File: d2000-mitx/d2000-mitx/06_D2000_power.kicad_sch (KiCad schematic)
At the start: 2 parts

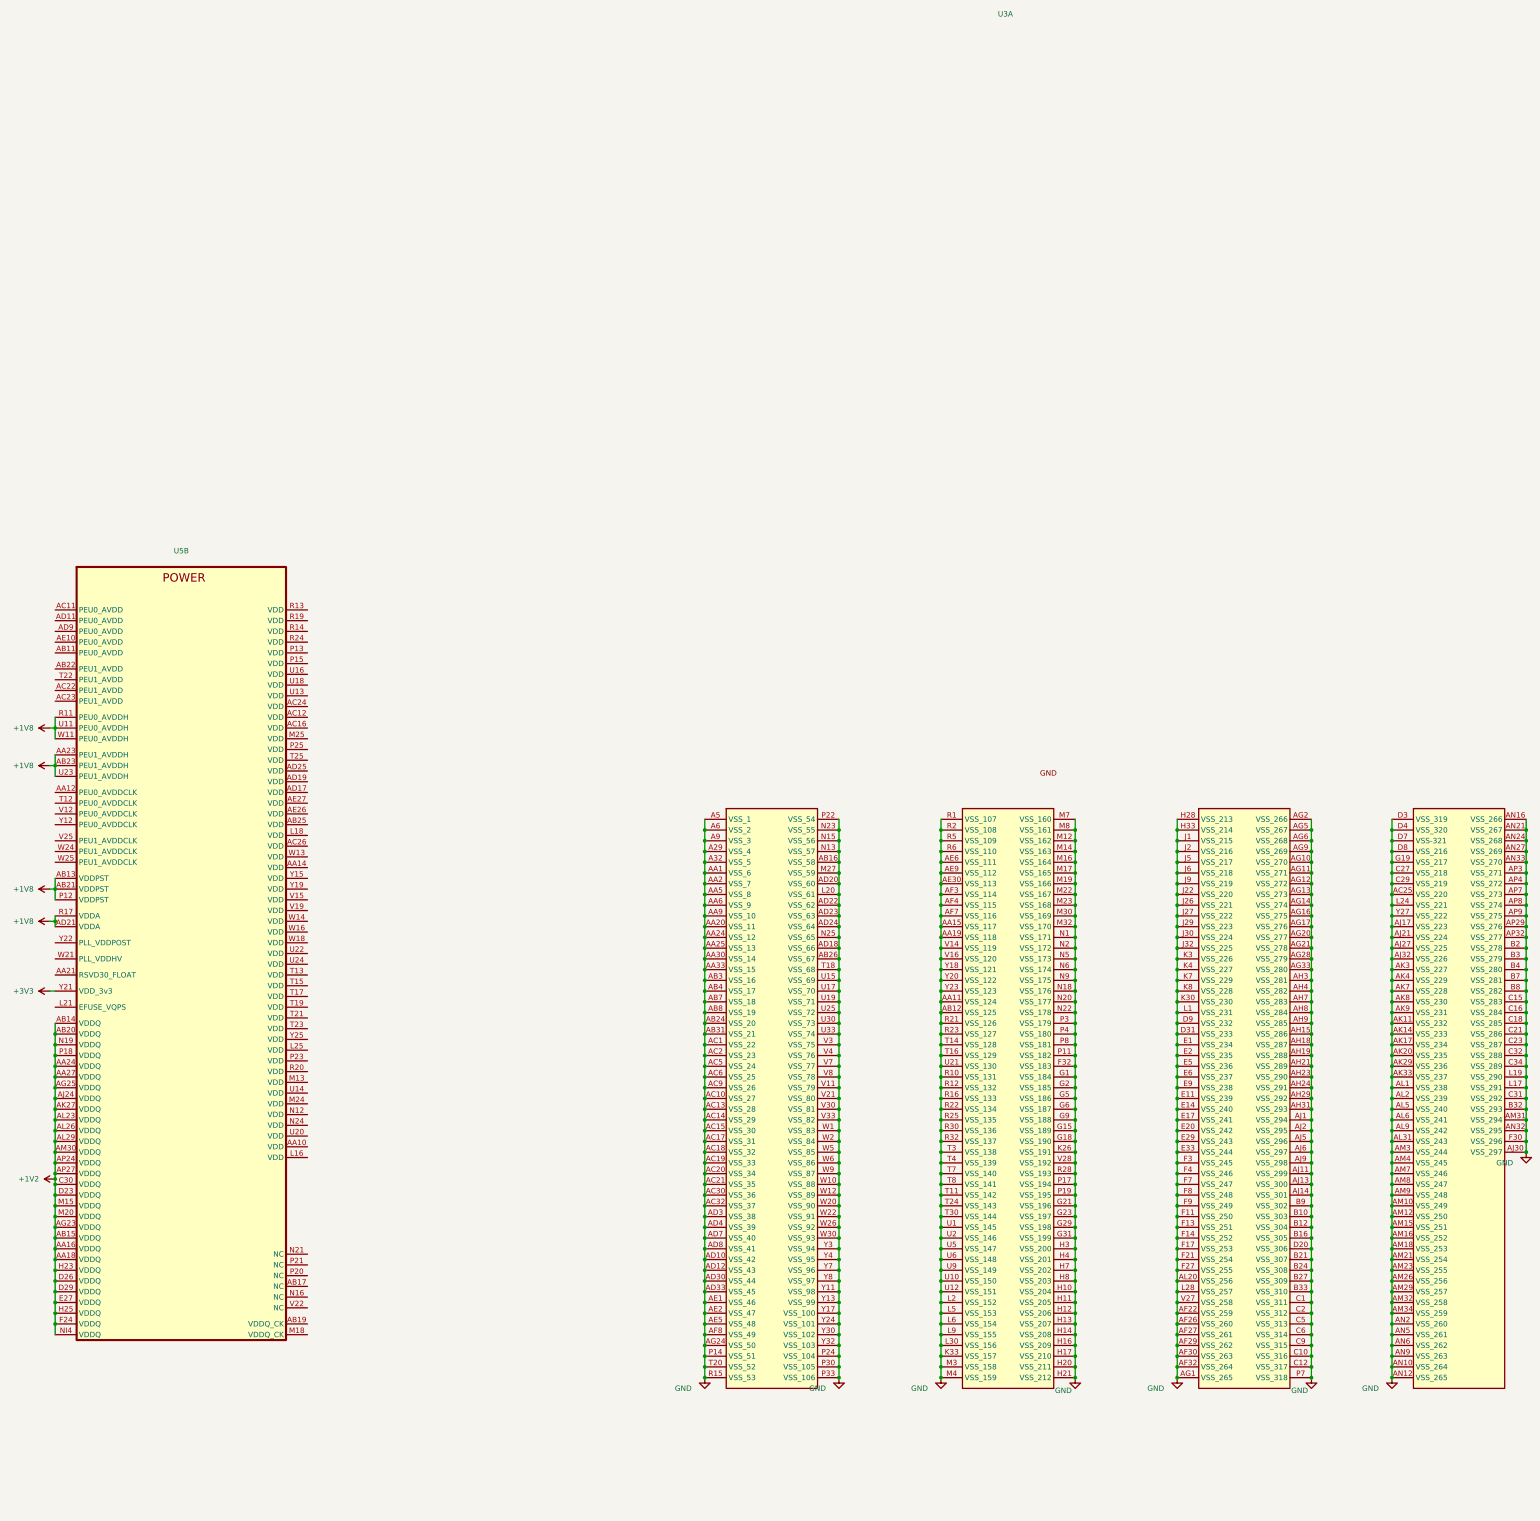
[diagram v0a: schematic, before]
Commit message: update schem + pcb layout
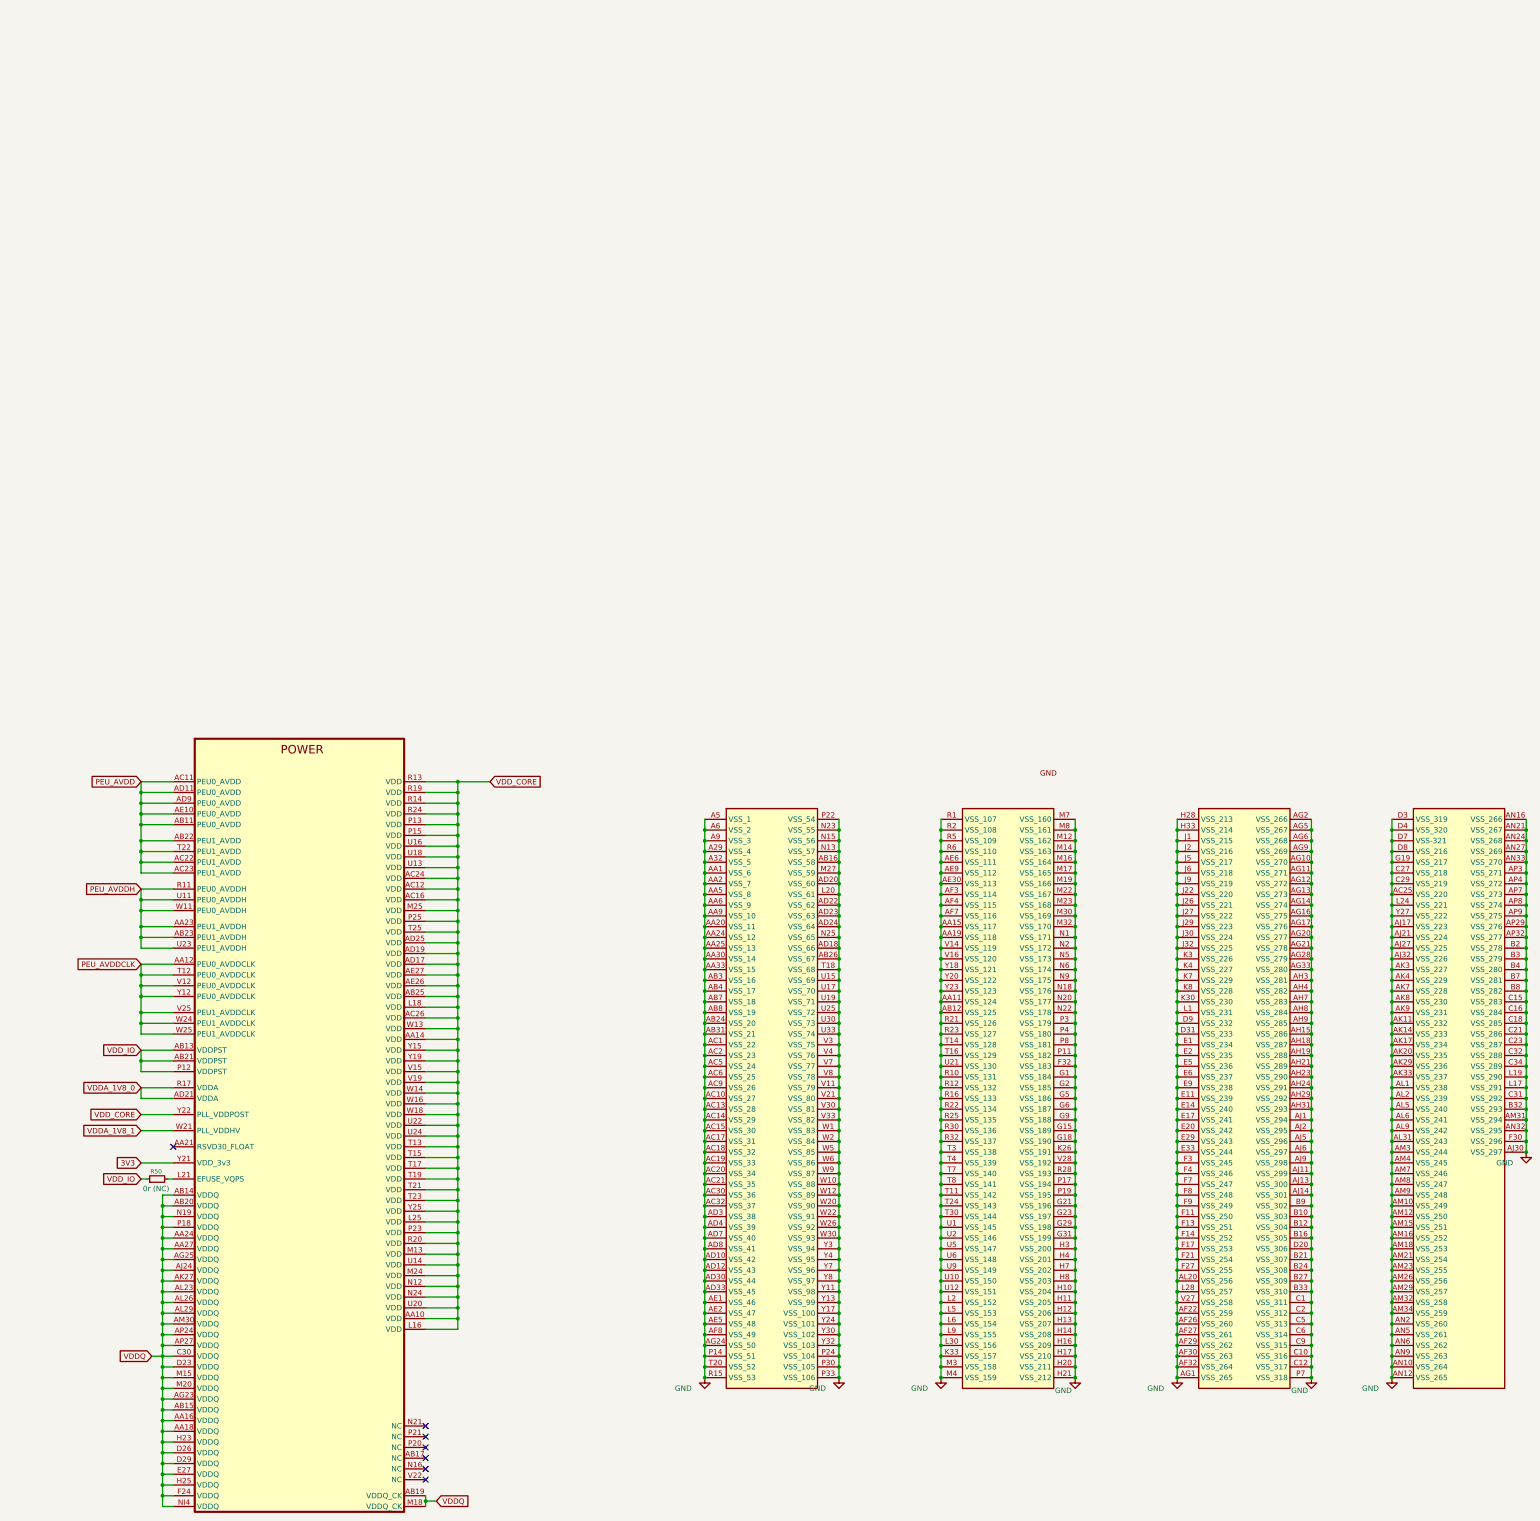
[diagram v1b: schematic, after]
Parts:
- removed U3, U5: ~, symbol D2000:D2000-E8
- added R50: 0r (NC), Resistor_SMD:R_0402_1005Metric, symbol Device:R_Small
- added U5: ~, D2000:D2000_DDR4_BGA1144P100_3500X350, symbol D2000-FT20004:D2000-E8
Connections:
- net GND: now also U5.A29 (VSS_4), U5.A32 (VSS_5), U5.A5 (VSS_1), U5.A6 (VSS_2), U5.A9 (VSS_3), U5.AA1 (VSS_6), U5.AA11 (VSS_124), U5.AA15 (VSS_117), U5.AA19 (VSS_118), U5.AA2 (VSS_7), U5.AA20 (VSS_11), U5.AA24 (VSS_12), U5.AA25 (VSS_13), U5.AA30 (VSS_14), U5.AA33 (VSS_15), U5.AA5 (VSS_8), U5.AA6 (VSS_9), U5.AA9 (VSS_10), U5.AB12 (VSS_125), U5.AB16 (VSS_58), U5.AB24 (VSS_20), U5.AB26 (VSS_67), U5.AB3 (VSS_16), U5.AB31 (VSS_21), U5.AB4 (VSS_17), U5.AB7 (VSS_18), U5.AB8 (VSS_19), U5.AC1 (VSS_22), U5.AC10 (VSS_27), U5.AC13 (VSS_28), U5.AC14 (VSS_29), U5.AC15 (VSS_30), U5.AC17 (VSS_31), U5.AC18 (VSS_32), U5.AC19 (VSS_33), U5.AC2 (VSS_23), U5.AC20 (VSS_34), U5.AC21 (VSS_35), U5.AC25 (VSS_220), U5.AC30 (VSS_36), U5.AC32 (VSS_37), U5.AC5 (VSS_24), U5.AC6 (VSS_25), U5.AC9 (VSS_26), U5.AD10 (VSS_42), U5.AD12 (VSS_43), U5.AD18 (VSS_66), U5.AD20 (VSS_60), U5.AD22 (VSS_62), U5.AD23 (VSS_63), U5.AD24 (VSS_64), U5.AD3 (VSS_38), U5.AD30 (VSS_44), U5.AD33 (VSS_45), U5.AD4 (VSS_39), U5.AD7 (VSS_40), U5.AD8 (VSS_41), U5.AE1 (VSS_46), U5.AE2 (VSS_47), U5.AE30 (VSS_113), U5.AE5 (VSS_48), U5.AE6 (VSS_111), U5.AE9 (VSS_112), U5.AF22 (VSS_259), U5.AF26 (VSS_260), U5.AF27 (VSS_261), U5.AF29 (VSS_262), U5.AF3 (VSS_114), U5.AF30 (VSS_263), U5.AF32 (VSS_264), U5.AF4 (VSS_115), U5.AF7 (VSS_116), U5.AF8 (VSS_49), U5.AG1 (VSS_265), U5.AG10 (VSS_270), U5.AG11 (VSS_271), U5.AG12 (VSS_272), U5.AG13 (VSS_273), U5.AG14 (VSS_274), U5.AG16 (VSS_275), U5.AG17 (VSS_276), U5.AG2 (VSS_266), U5.AG20 (VSS_277), U5.AG21 (VSS_278), U5.AG24 (VSS_50), U5.AG28 (VSS_279), U5.AG33 (VSS_280), U5.AG5 (VSS_267), U5.AG6 (VSS_268), U5.AG9 (VSS_269), U5.AH15 (VSS_286), U5.AH18 (VSS_287), U5.AH19 (VSS_288), U5.AH21 (VSS_289), U5.AH23 (VSS_290), U5.AH24 (VSS_291), U5.AH29 (VSS_292), U5.AH3 (VSS_281), U5.AH31 (VSS_293), U5.AH4 (VSS_282), U5.AH7 (VSS_283), U5.AH8 (VSS_284), U5.AH9 (VSS_285), U5.AJ1 (VSS_294), U5.AJ11 (VSS_299), U5.AJ13 (VSS_300), U5.AJ14 (VSS_301), U5.AJ17 (VSS_223), U5.AJ2 (VSS_295), U5.AJ21 (VSS_224), U5.AJ27 (VSS_225), U5.AJ30 (VSS_297), U5.AJ32 (VSS_226), U5.AJ5 (VSS_296), U5.AJ6 (VSS_297), U5.AJ9 (VSS_298), U5.AK11 (VSS_232), U5.AK14 (VSS_233), U5.AK17 (VSS_234), U5.AK20 (VSS_235), U5.AK29 (VSS_236), U5.AK3 (VSS_227), U5.AK33 (VSS_237), U5.AK4 (VSS_229), U5.AK7 (VSS_228), U5.AK8 (VSS_230), U5.AK9 (VSS_231), U5.AL1 (VSS_238), U5.AL2 (VSS_239), U5.AL20 (VSS_256), U5.AL31 (VSS_243), U5.AL5 (VSS_240), U5.AL6 (VSS_241), U5.AL9 (VSS_242), U5.AM10 (VSS_249), U5.AM12 (VSS_250), U5.AM15 (VSS_251), U5.AM16 (VSS_252), U5.AM18 (VSS_253), U5.AM21 (VSS_254), U5.AM23 (VSS_255), U5.AM26 (VSS_256), U5.AM29 (VSS_257), U5.AM3 (VSS_244), U5.AM31 (VSS_294), U5.AM32 (VSS_258), U5.AM34 (VSS_259), U5.AM4 (VSS_245), U5.AM7 (VSS_246), U5.AM8 (VSS_247), U5.AM9 (VSS_248), U5.AN10 (VSS_264), U5.AN12 (VSS_265), U5.AN16 (VSS_266), U5.AN2 (VSS_260), U5.AN21 (VSS_267), U5.AN24 (VSS_268), U5.AN27 (VSS_269), U5.AN32 (VSS_295), U5.AN33 (VSS_270), U5.AN5 (VSS_261), U5.AN6 (VSS_262), U5.AN9 (VSS_263), U5.AP29 (VSS_276), U5.AP3 (VSS_271), U5.AP32 (VSS_277), U5.AP4 (VSS_272), U5.AP7 (VSS_273), U5.AP8 (VSS_274), U5.AP9 (VSS_275), U5.B10 (VSS_303), U5.B12 (VSS_304), U5.B16 (VSS_305), U5.B2 (VSS_278), U5.B21 (VSS_307), U5.B24 (VSS_308), U5.B27 (VSS_309), U5.B3 (VSS_279), U5.B32 (VSS_293), U5.B33 (VSS_310), U5.B4 (VSS_280), U5.B7 (VSS_281), U5.B8 (VSS_282), U5.B9 (VSS_302), U5.C1 (VSS_311), U5.C10 (VSS_316), U5.C12 (VSS_317), U5.C15 (VSS_283), U5.C16 (VSS_284), U5.C18 (VSS_285), U5.C2 (VSS_312), U5.C21 (VSS_286), U5.C23 (VSS_287), U5.C27 (VSS_218), U5.C29 (VSS_219), U5.C31 (VSS_292), U5.C32 (VSS_288), U5.C34 (VSS_289), U5.C5 (VSS_313), U5.C6 (VSS_314), U5.C9 (VSS_315), U5.D20 (VSS_306), U5.D3 (VSS_319), U5.D31 (VSS_233), U5.D4 (VSS_320), U5.D7 (VSS-321), U5.D8 (VSS_216), U5.D9 (VSS_232), U5.E1 (VSS_234), U5.E11 (VSS_239), U5.E14 (VSS_240), U5.E17 (VSS_241), U5.E2 (VSS_235), U5.E20 (VSS_242), U5.E29 (VSS_243), U5.E33 (VSS_244), U5.E5 (VSS_236), U5.E6 (VSS_237), U5.E9 (VSS_238), U5.F11 (VSS_250), U5.F13 (VSS_251), U5.F14 (VSS_252), U5.F17 (VSS_253), U5.F21 (VSS_254), U5.F27 (VSS_255), U5.F3 (VSS_245), U5.F30 (VSS_296), U5.F32 (VSS_183), U5.F4 (VSS_246), U5.F7 (VSS_247), U5.F8 (VSS_248), U5.F9 (VSS_249), U5.G1 (VSS_184), U5.G15 (VSS_189), U5.G18 (VSS_190), U5.G19 (VSS_217), U5.G2 (VSS_185), U5.G21 (VSS_196), U5.G23 (VSS_197), U5.G29 (VSS_198), U5.G31 (VSS_199), U5.G5 (VSS_186), U5.G6 (VSS_187), U5.G9 (VSS_188), U5.H10 (VSS_204), U5.H11 (VSS_205), U5.H12 (VSS_206), U5.H13 (VSS_207), U5.H14 (VSS_208), U5.H16 (VSS_209), U5.H17 (VSS_210), U5.H20 (VSS_211), U5.H21 (VSS_212), U5.H28 (VSS_213), U5.H3 (VSS_200), U5.H33 (VSS_214), U5.H4 (VSS_201), U5.H7 (VSS_202), U5.H8 (VSS_203), U5.J1 (VSS_215), U5.J2 (VSS_216), U5.J22 (VSS_220), U5.J26 (VSS_221), U5.J27 (VSS_222), U5.J29 (VSS_223), U5.J30 (VSS_224), U5.J32 (VSS_225), U5.J5 (VSS_217), U5.J6 (VSS_218), U5.J9 (VSS_219), U5.K26 (VSS_191), U5.K3 (VSS_226), U5.K30 (VSS_230), U5.K33 (VSS_157), U5.K4 (VSS_227), U5.K7 (VSS_229), U5.K8 (VSS_228), U5.L1 (VSS_231), U5.L17 (VSS_291), U5.L19 (VSS_290), U5.L2 (VSS_152), U5.L20 (VSS_61), U5.L24 (VSS_221), U5.L28 (VSS_257), U5.L30 (VSS_156), U5.L5 (VSS_153), U5.L6 (VSS_154), U5.L9 (VSS_155), U5.M12 (VSS_162), U5.M14 (VSS_163), U5.M16 (VSS_164), U5.M17 (VSS_165), U5.M19 (VSS_166), U5.M22 (VSS_167), U5.M23 (VSS_168), U5.M27 (VSS_59), U5.M3 (VSS_158), U5.M30 (VSS_169), U5.M32 (VSS_170), U5.M4 (VSS_159), U5.M7 (VSS_160), U5.M8 (VSS_161), U5.N1 (VSS_171), U5.N13 (VSS_57), U5.N15 (VSS_56), U5.N18 (VSS_176), U5.N2 (VSS_172), U5.N20 (VSS_177), U5.N22 (VSS_178), U5.N23 (VSS_55), U5.N25 (VSS_65), U5.N5 (VSS_173), U5.N6 (VSS_174), U5.N9 (VSS_175), U5.P11 (VSS_182), U5.P14 (VSS_51), U5.P17 (VSS_194), U5.P19 (VSS_195), U5.P22 (VSS_54), U5.P24 (VSS_104), U5.P3 (VSS_179), U5.P30 (VSS_105), U5.P33 (VSS_106), U5.P4 (VSS_180), U5.P7 (VSS_318), U5.P8 (VSS_181), U5.R1 (VSS_107), U5.R10 (VSS_131), U5.R12 (VSS_132), U5.R15 (VSS_53), U5.R16 (VSS_133), U5.R2 (VSS_108), U5.R21 (VSS_126), U5.R22 (VSS_134), U5.R23 (VSS_127), U5.R25 (VSS_135), U5.R28 (VSS_193), U5.R30 (VSS_136), U5.R32 (VSS_137), U5.R5 (VSS_109), U5.R6 (VSS_110), U5.T11 (VSS_142), U5.T14 (VSS_128), U5.T16 (VSS_129), U5.T18 (VSS_68), U5.T20 (VSS_52), U5.T24 (VSS_143), U5.T3 (VSS_138), U5.T30 (VSS_144), U5.T4 (VSS_139), U5.T7 (VSS_140), U5.T8 (VSS_141), U5.U1 (VSS_145), U5.U10 (VSS_150), U5.U12 (VSS_151), U5.U15 (VSS_69), U5.U17 (VSS_70), U5.U19 (VSS_71), U5.U2 (VSS_146), U5.U21 (VSS_130), U5.U25 (VSS_72), U5.U30 (VSS_73), U5.U33 (VSS_74), U5.U5 (VSS_147), U5.U6 (VSS_148), U5.U9 (VSS_149), U5.V11 (VSS_79), U5.V14 (VSS_119), U5.V16 (VSS_120), U5.V21 (VSS_80), U5.V27 (VSS_258), U5.V28 (VSS_192), U5.V3 (VSS_75), U5.V30 (VSS_81), U5.V33 (VSS_82), U5.V4 (VSS_76), U5.V7 (VSS_77), U5.V8 (VSS_78), U5.W1 (VSS_83), U5.W10 (VSS_88), U5.W12 (VSS_89), U5.W2 (VSS_84), U5.W20 (VSS_90), U5.W22 (VSS_91), U5.W26 (VSS_92), U5.W30 (VSS_93), U5.W5 (VSS_85), U5.W6 (VSS_86), U5.W9 (VSS_87), U5.Y11 (VSS_98), U5.Y13 (VSS_99), U5.Y17 (VSS_100), U5.Y18 (VSS_121), U5.Y20 (VSS_122), U5.Y23 (VSS_123), U5.Y24 (VSS_101), U5.Y27 (VSS_222), U5.Y3 (VSS_94), U5.Y30 (VSS_102), U5.Y32 (VSS_103)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
- new net: R50.2, U5.L21 (EFUSE_VQPS)
- new net 3V3: U5.Y21 (VDD_3v3)
- new net PEU_AVDD: U5.AB11 (PEU0_AVDD), U5.AB22 (PEU1_AVDD), U5.AC11 (PEU0_AVDD), U5.AC22 (PEU1_AVDD), U5.AC23 (PEU1_AVDD), U5.AD11 (PEU0_AVDD), U5.AD9 (PEU0_AVDD), U5.AE10 (PEU0_AVDD), U5.T22 (PEU1_AVDD)
- new net PEU_AVDDCLK: U5.AA12 (PEU0_AVDDCLK), U5.T12 (PEU0_AVDDCLK), U5.V12 (PEU0_AVDDCLK), U5.V25 (PEU1_AVDDCLK), U5.W24 (PEU1_AVDDCLK), U5.W25 (PEU1_AVDDCLK), U5.Y12 (PEU0_AVDDCLK)
- new net PEU_AVDDH: U5.AA23 (PEU1_AVDDH), U5.AB23 (PEU1_AVDDH), U5.R11 (PEU0_AVDDH), U5.U11 (PEU0_AVDDH), U5.U23 (PEU1_AVDDH), U5.W11 (PEU0_AVDDH)
- new net VDDA_1V8_0: U5.AD21 (VDDA), U5.R17 (VDDA)
- new net VDDA_1V8_1: U5.W21 (PLL_VDDHV)
- new net VDDQ: U5.AA16 (VDDQ), U5.AA18 (VDDQ), U5.AA24 (VDDQ), U5.AA27 (VDDQ), U5.AB14 (VDDQ), U5.AB15 (VDDQ), U5.AB19 (VDDQ_CK), U5.AB20 (VDDQ), U5.AG23 (VDDQ), U5.AG25 (VDDQ), U5.AJ24 (VDDQ), U5.AK27 (VDDQ), U5.AL23 (VDDQ), U5.AL26 (VDDQ), U5.AL29 (VDDQ), U5.AM30 (VDDQ), U5.AP24 (VDDQ), U5.AP27 (VDDQ), U5.C30 (VDDQ), U5.D23 (VDDQ), U5.D26 (VDDQ), U5.D29 (VDDQ), U5.E27 (VDDQ), U5.F24 (VDDQ), U5.H23 (VDDQ), U5.H25 (VDDQ), U5.M15 (VDDQ), U5.M18 (VDDQ_CK), U5.M20 (VDDQ), U5.N19 (VDDQ), U5.NI4 (VDDQ), U5.P18 (VDDQ)
- new net VDD_CORE: U5.AA10 (VDD), U5.AA14 (VDD), U5.AB25 (VDD), U5.AC12 (VDD), U5.AC16 (VDD), U5.AC24 (VDD), U5.AC26 (VDD), U5.AD17 (VDD), U5.AD19 (VDD), U5.AD25 (VDD), U5.AE26 (VDD), U5.AE27 (VDD), U5.L16 (VDD), U5.L18 (VDD), U5.L25 (VDD), U5.M13 (VDD), U5.M24 (VDD), U5.M25 (VDD), U5.N12 (VDD), U5.N24 (VDD), U5.P13 (VDD), U5.P15 (VDD), U5.P23 (VDD), U5.P25 (VDD), U5.R13 (VDD), U5.R14 (VDD), U5.R19 (VDD), U5.R20 (VDD), U5.R24 (VDD), U5.T13 (VDD), U5.T15 (VDD), U5.T17 (VDD), U5.T19 (VDD), U5.T21 (VDD), U5.T23 (VDD), U5.T25 (VDD), U5.U13 (VDD), U5.U14 (VDD), U5.U16 (VDD), U5.U18 (VDD), U5.U20 (VDD), U5.U22 (VDD), U5.U24 (VDD), U5.V15 (VDD), U5.V19 (VDD), U5.W13 (VDD), U5.W14 (VDD), U5.W16 (VDD), U5.W18 (VDD), U5.Y15 (VDD), U5.Y19 (VDD), U5.Y22 (PLL_VDDPOST), U5.Y25 (VDD)
- new net VDD_IO: R50.1, U5.AB13 (VDDPST), U5.AB21 (VDDPST), U5.P12 (VDDPST)
- no-connect marks 0 -> 7
